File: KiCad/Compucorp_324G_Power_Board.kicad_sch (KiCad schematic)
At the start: 5 parts, among them J7 Power Interboard, J8 Power In, J9 To Scan Board

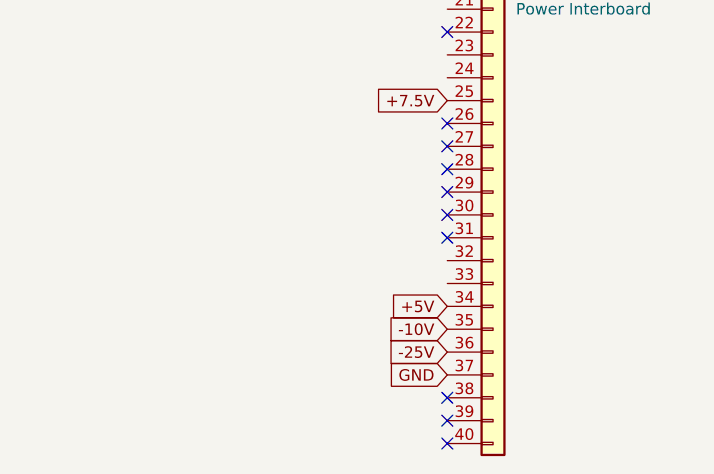
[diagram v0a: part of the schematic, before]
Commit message: Memory board updates
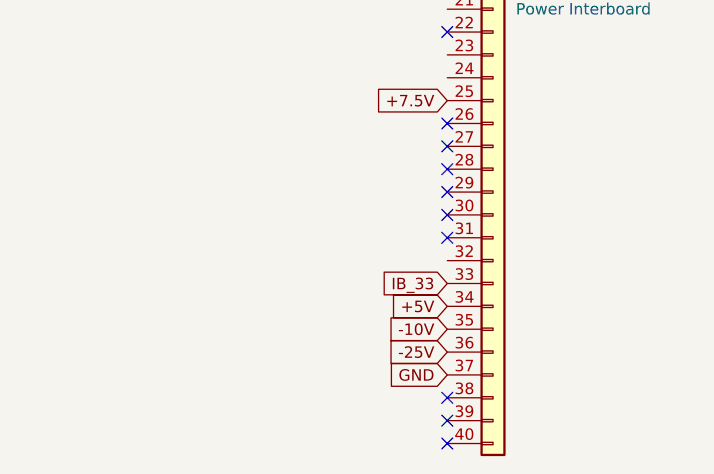
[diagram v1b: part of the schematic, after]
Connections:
- net IB_33: now reaches J7.33 (Pin_33)
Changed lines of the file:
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@@
+		)
+	)
+	(global_label "IB_33"
+		(shape input)
+		(at 243.84 121.92 180)
+		(fields_autoplaced yes)
+		(effects
+			(font
+				(size 1.27 1.27)
+			)
+			(justify right)
+		)
+		(property "Intersheetrefs" "${INTERSHEET_REFS}"
+			(at 235.5934 121.92 0)
+			(effects
+				(font
+					(size 1.27 1.27)
+				)
+				(justify right)
+				(hide yes)
+			)
 		)
 	)

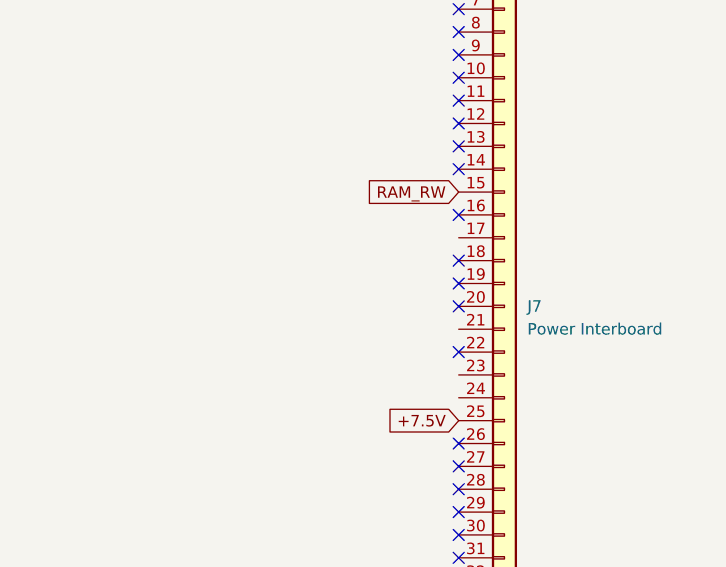
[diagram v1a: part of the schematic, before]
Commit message: Memory board updates
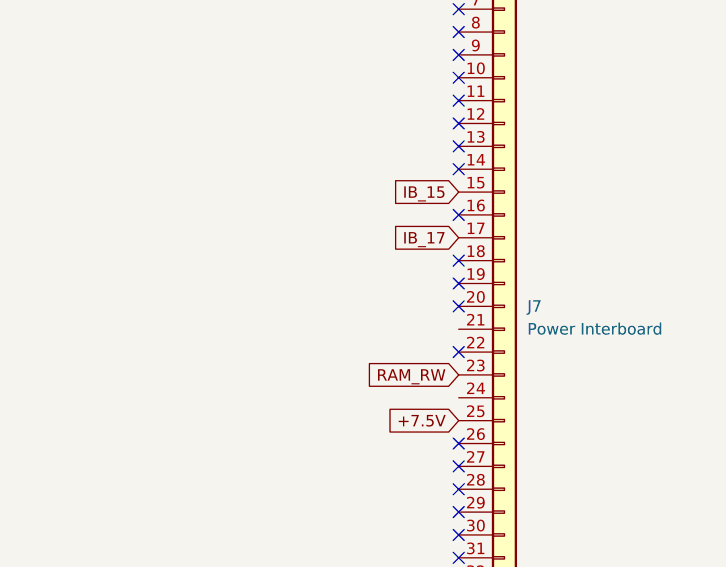
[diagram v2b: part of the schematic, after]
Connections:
- net RAM_RW: now also J7.23 (Pin_23); no longer J7.15 (Pin_15)
- net IB_17: now reaches J7.17 (Pin_17)
- new net IB_15: J7.15 (Pin_15)
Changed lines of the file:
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@@
+		)
+	)
+	(global_label "IB_15"
+		(shape input)
+		(at 243.84 76.2 180)
+		(fields_autoplaced yes)
+		(effects
+			(font
+				(size 1.27 1.27)
+			)
+			(justify right)
+		)
+		(property "Intersheetrefs" "${INTERSHEET_REFS}"
+			(at 235.5934 76.2 0)
+			(effects
+				(font
+					(size 1.27 1.27)
+				)
+				(justify right)
+				(hide yes)
+			)
 		)
 	)
@@
 		)
 	)
+	(global_label "+7.5V"
+		(shape input)
+		(at 157.48 124.46 180)
+		(fields_autoplaced yes)
+		(effects
+			(font
+				(size 1.27 1.27)
+			)
+			(justify right)
+		)
+		(property "Intersheetrefs" "${INTERSHEET_REFS}"
+			(at 148.81 124.46 0)
+			(effects
+				(font
+					(size 1.27 1.27)
+				)
+				(justify right)
+				(hide yes)
+			)
+		)
+	)
+	(global_label "-10V"
+		(shape input)
+		(at 243.84 127 180)
+		(fields_autoplaced yes)
+		(effects
+			(font
+				(size 1.27 1.27)
+			)
+			(justify right)
+		)
+		(property "Intersheetrefs" "${INTERSHEET_REFS}"
+			(at 235.7748 127 0)
+			(effects
+				(font
+					(size 1.27 1.27)
+				)
+				(justify right)
+				(hide yes)
+			)
+		)
+	)
+	(global_label "+5V"
+		(shape input)
+		(at 157.48 114.3 180)
+		(fields_autoplaced yes)
+		(effects
+			(font
+				(size 1.27 1.27)
+			)
+			(justify right)
+		)
+		(property "Intersheetrefs" "${INTERSHEET_REFS}"
+			(at 150.6243 114.3 0)
+			(effects
+				(font
+					(size 1.27 1.27)
+				)
+				(justify right)
+				(hide yes)
+			)
+		)
+	)
+	(global_label "+5V"
+		(shape input)
+		(at 243.84 124.46 180)
+		(fields_autoplaced yes)
+		(effects
+			(font
+				(size 1.27 1.27)
+			)
+			(justify right)
+		)
+		(property "Intersheetrefs" "${INTERSHEET_REFS}"
+			(at 236.9843 124.46 0)
+			(effects
+				(font
+					(size 1.27 1.27)
+				)
+				(justify right)
+				(hide yes)
+			)
+		)
+	)
+	(global_label "IB_17"
+		(shape input)
+		(at 243.84 81.28 180)
+		(fields_autoplaced yes)
+		(effects
+			(font
+				(size 1.27 1.27)
+			)
+			(justify right)
+		)
+		(property "Intersheetrefs" "${INTERSHEET_REFS}"
+			(at 235.5934 81.28 0)
+			(effects
+				(font
+					(size 1.27 1.27)
+				)
+				(justify right)
+				(hide yes)
+			)
+		)
+	)
+	(global_label "+7.5V"
+		(shape input)
+		(at 243.84 101.6 180)
+		(fields_autoplaced yes)
+		(effects
+			(font
+				(size 1.27 1.27)
+			)
+			(justify right)
+		)
+		(property "Intersheetrefs" "${INTERSHEET_REFS}"
+			(at 235.17 101.6 0)
+			(effects
+				(font
+					(size 1.27 1.27)
+				)
+				(justify right)
+				(hide yes)
+			)
+		)
+	)
+	(global_label "GND"
+		(shape input)
+		(at 243.84 132.08 180)
+		(fields_autoplaced yes)
+		(effects
+			(font
+				(size 1.27 1.27)
+			)
+			(justify right)
+		)
+		(property "Intersheetrefs" "${INTERSHEET_REFS}"
+			(at 236.9843 132.08 0)
+			(effects
+				(font
+					(size 1.27 1.27)
+				)
+				(justify right)
+				(hide yes)
+			)
+		)
+	)
 	(global_label "RAM_RW"
 		(shape input)
-		(at 243.84 76.2 180)
-		(fields_autoplaced yes)
-		(effects
-			(font
-				(size 1.27 1.27)
-			)
-			(justify right)
-		)
-		(property "Intersheetrefs" "${INTERSHEET_REFS}"
-			(at 233.3558 76.2 0)
-			(effects
-				(font
-					(size 1.27 1.27)
-				)
-				(justify right)
-				(hide yes)
-			)
-		)
-	)
-	(global_label "+7.5V"
-		(shape input)
-		(at 157.48 124.46 180)
-		(fields_autoplaced yes)
-		(effects
-			(font
-				(size 1.27 1.27)
-			)
-			(justify right)
-		)
-		(property "Intersheetrefs" "${INTERSHEET_REFS}"
-			(at 148.81 124.46 0)
-			(effects
-				(font
-					(size 1.27 1.27)
-				)
-				(justify right)
-				(hide yes)
-			)
-		)
-	)
-	(global_label "-10V"
-		(shape input)
-		(at 243.84 127 180)
-		(fields_autoplaced yes)
-		(effects
-			(font
-				(size 1.27 1.27)
-			)
-			(justify right)
-		)
-		(property "Intersheetrefs" "${INTERSHEET_REFS}"
-			(at 235.7748 127 0)
-			(effects
-				(font
-					(size 1.27 1.27)
-				)
-				(justify right)
-				(hide yes)
-			)
-		)
-	)
-	(global_label "+5V"
-		(shape input)
-		(at 157.48 114.3 180)
-		(fields_autoplaced yes)
-		(effects
-			(font
-				(size 1.27 1.27)
-			)
-			(justify right)
-		)
-		(property "Intersheetrefs" "${INTERSHEET_REFS}"
-			(at 150.6243 114.3 0)
-			(effects
-				(font
-					(size 1.27 1.27)
-				)
-				(justify right)
-				(hide yes)
-			)
-		)
-	)
-	(global_label "+5V"
-		(shape input)
-		(at 243.84 124.46 180)
-		(fields_autoplaced yes)
-		(effects
-			(font
-				(size 1.27 1.27)
-			)
-			(justify right)
-		)
-		(property "Intersheetrefs" "${INTERSHEET_REFS}"
-			(at 236.9843 124.46 0)
-			(effects
-				(font
-					(size 1.27 1.27)
-				)
-				(justify right)
-				(hide yes)
-			)
-		)
-	)
-	(global_label "+7.5V"
-		(shape input)
-		(at 243.84 101.6 180)
-		(fields_autoplaced yes)
-		(effects
-			(font
-				(size 1.27 1.27)
-			)
-			(justify right)
-		)
-		(property "Intersheetrefs" "${INTERSHEET_REFS}"
-			(at 235.17 101.6 0)
-			(effects
-				(font
-					(size 1.27 1.27)
-				)
-				(justify right)
-				(hide yes)
-			)
-		)
-	)
-	(global_label "GND"
-		(shape input)
-		(at 243.84 132.08 180)
-		(fields_autoplaced yes)
-		(effects
-			(font
-				(size 1.27 1.27)
-			)
-			(justify right)
-		)
-		(property "Intersheetrefs" "${INTERSHEET_REFS}"
-			(at 236.9843 132.08 0)
-			(effects
-				(font
+		(at 243.84 96.52 180)
+		(fields_autoplaced yes)
+		(effects
+			(font
+				(size 1.27 1.27)
+			)
+			(justify right)
+		)
+		(property "Intersheetrefs" "${INTERSHEET_REFS}"
+			(at 233.3558 96.52 0)
+			(effects
+				(font
